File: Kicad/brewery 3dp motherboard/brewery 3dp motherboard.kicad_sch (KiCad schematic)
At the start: 33 parts, among them J1 power in, J16 heater in, SW1 SW_Push, SW2 SW_Push, U14 STM32F407Z_E-G_Tx

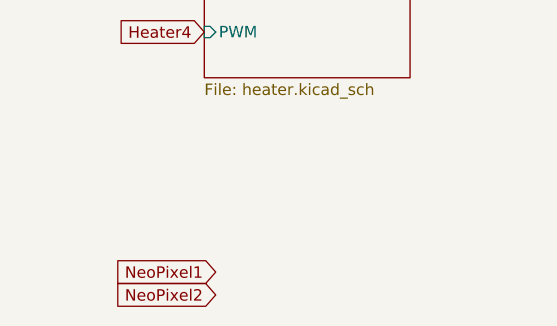
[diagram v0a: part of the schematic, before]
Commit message: stufffff
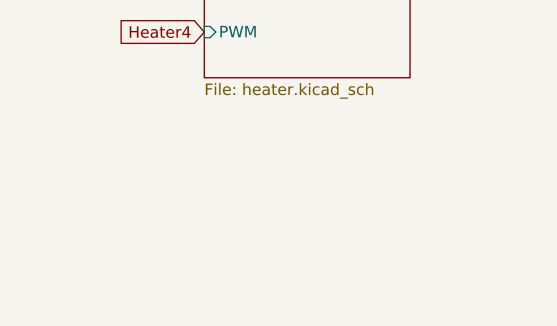
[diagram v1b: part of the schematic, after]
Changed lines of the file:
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@@
-		)
-	)
-	(global_label "NeoPixel2"
-		(shape input)
-		(at 34.29 264.16 180)
-		(fields_autoplaced yes)
-		(effects
-			(font
-				(size 1.27 1.27)
-			)
-			(justify right)
-		)
-		(property "Intersheetrefs" "${INTERSHEET_REFS}"
-			(at 21.8705 264.16 0)
-			(hide yes)
-			(show_name no)
-			(do_not_autoplace no)
-			(effects
-				(font
-					(size 1.27 1.27)
-				)
-				(justify right)
-			)
 		)
 	)
@@
 			)
 		)
-	)
-	(global_label "NeoPixel1"
-		(shape input)
-		(at 34.29 261.62 180)
-		(fields_autoplaced yes)
-		(effects
-			(font
-				(size 1.27 1.27)
-			)
-			(justify right)
-		)
-		(property "Intersheetrefs" "${INTERSHEET_REFS}"
-			(at 21.8705 261.62 0)
-			(hide yes)
-			(show_name no)
-			(do_not_autoplace no)
-			(effects
-				(font
-					(size 1.27 1.27)
-				)
-				(justify right)
-			)
-		)
